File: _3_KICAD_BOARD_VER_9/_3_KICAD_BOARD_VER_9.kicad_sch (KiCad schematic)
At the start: 0 parts

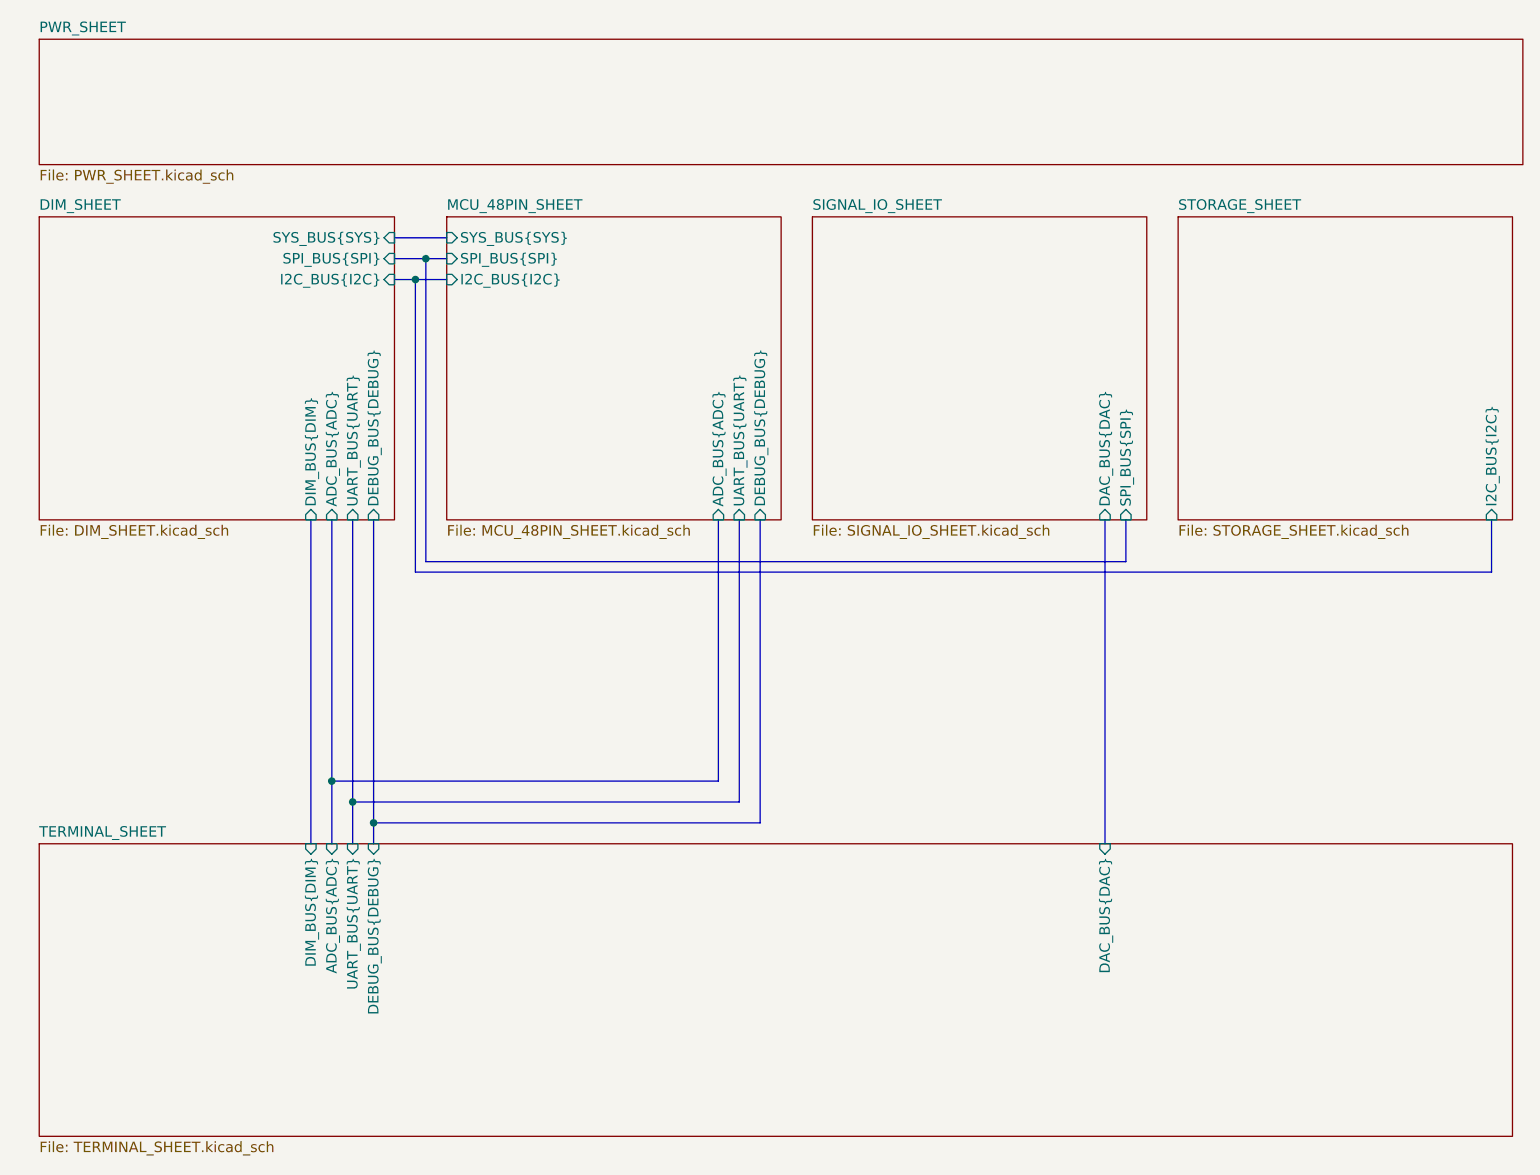
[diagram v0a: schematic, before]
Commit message: feat : dim only project done
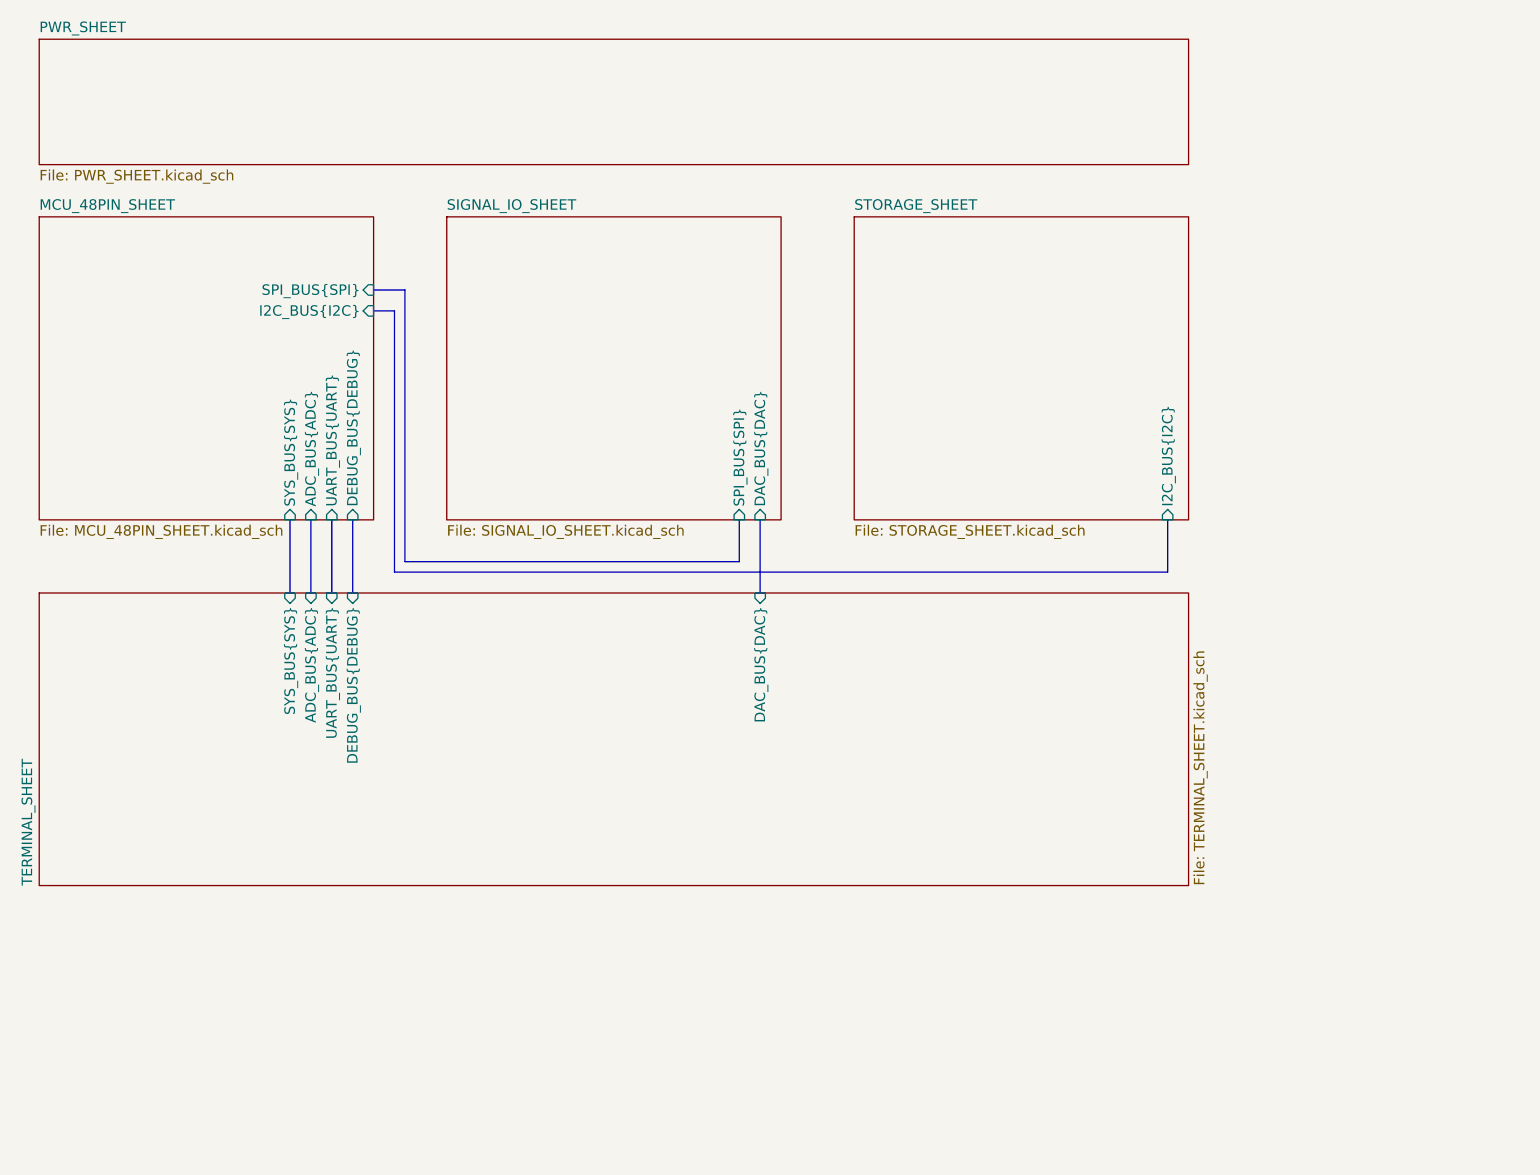
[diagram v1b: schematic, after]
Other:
- removed sheet DIM_SHEET
- sheet TERMINAL_SHEET ports: added SYS_BUS{SYS}; removed DIM_BUS{DIM}
